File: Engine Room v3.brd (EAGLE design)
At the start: 72.4 x 35.6 mm, 28 parts, among them Q201 IRF6718, Q202 IRF6718, U101 PC847, U201 L298

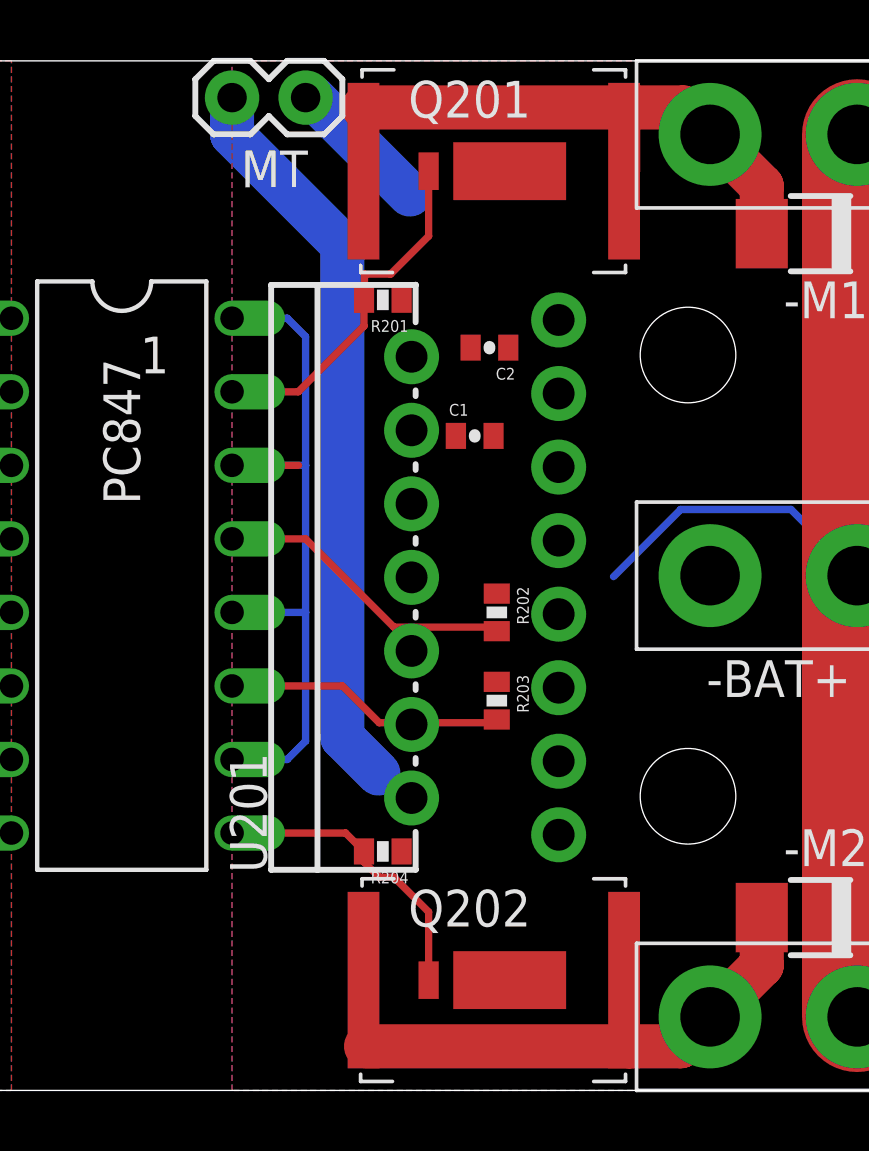
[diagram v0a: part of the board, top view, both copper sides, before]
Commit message: Added KwanAstro after the little crash of 2012
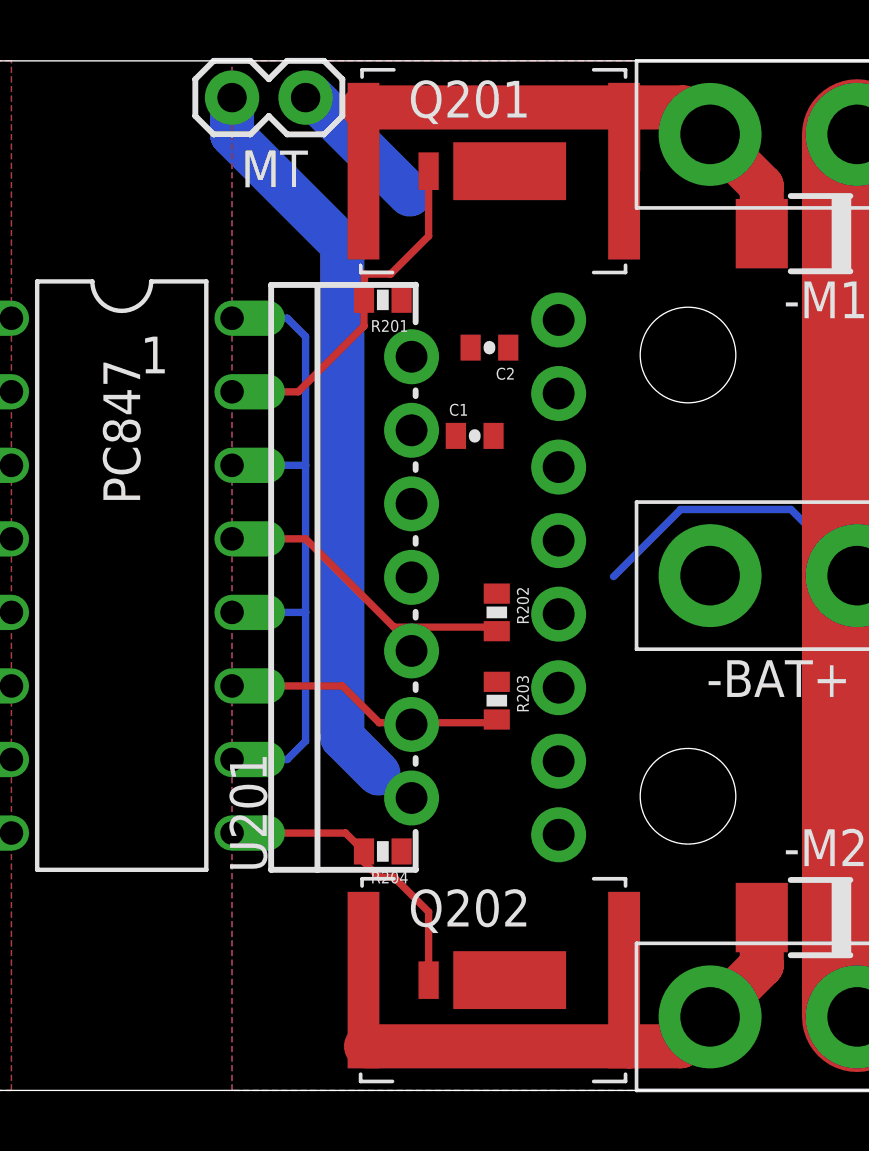
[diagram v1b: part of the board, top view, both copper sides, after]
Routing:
- net VDD: track 74.4 -> 72.1 mm
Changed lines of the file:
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@@
 <wire x1="64.77" y1="33.02" x2="66.555" y2="31.235" width="1.524" layer="1"/>
 <wire x1="66.555" y1="31.235" x2="66.555" y2="29.591" width="1.524" layer="1"/>
+<wire x1="63.84" y1="33.95" x2="62.23" y2="33.95" width="1.524" layer="1"/>
+<wire x1="62.23" y1="33.95" x2="52.8" y2="33.95" width="1.524" layer="1"/>
+<wire x1="62.23" y1="31.75" x2="62.23" y2="33.95" width="0.254" layer="1"/>
 <contactref element="Q201" pad="D1"/>
 <contactref element="Q201" pad="D2"/>
-<wire x1="63.84" y1="33.95" x2="62.23" y2="33.95" width="1.524" layer="1"/>
-<wire x1="62.23" y1="33.95" x2="52.8" y2="33.95" width="1.524" layer="1"/>
-<wire x1="52.8" y1="33.95" x2="52.8" y2="31.75" width="0.254" layer="1"/>
-<wire x1="61.8" y1="31.75" x2="62.23" y2="31.75" width="0.254" layer="1"/>
-<wire x1="62.23" y1="31.75" x2="62.23" y2="33.95" width="0.254" layer="1"/>
+<wire x1="52.8" y1="33.95" x2="53.34" y2="33.95" width="0.254" layer="1"/>
+<wire x1="53.34" y1="33.95" x2="53.34" y2="34.29" width="0.254" layer="1"/>
+<wire x1="52.8" y1="31.75" x2="52.8" y2="33.95" width="0.254" layer="1"/>
+<wire x1="62.23" y1="31.75" x2="61.8" y2="31.75" width="0" layer="19" extent="1-1"/>
 </signal>
 <signal name="M2-" class="1">
@@
 <wire x1="64.77" y1="2.54" x2="66.555" y2="4.325" width="1.524" layer="1"/>
 <wire x1="66.555" y1="4.325" x2="66.555" y2="5.969" width="1.524" layer="1"/>
+<wire x1="52.886" y1="1.524" x2="52.8" y2="1.524" width="0.254" layer="1"/>
+<wire x1="61.89" y1="3.81" x2="61.89" y2="1.61" width="0.254" layer="1"/>
 <contactref element="Q202" pad="D1"/>
 <contactref element="Q202" pad="D2"/>
-<wire x1="52.886" y1="1.524" x2="52.8" y2="1.524" width="0.254" layer="1"/>
 <wire x1="52.8" y1="1.524" x2="52.8" y2="3.81" width="0.254" layer="1"/>
-<wire x1="61.8" y1="3.81" x2="61.89" y2="3.81" width="0.254" layer="1"/>
-<wire x1="61.89" y1="3.81" x2="61.89" y2="1.61" width="0.254" layer="1"/>
+<wire x1="61.89" y1="3.81" x2="61.8" y2="3.81" width="0" layer="19" extent="1-1"/>
 </signal>
 <signal name="VDD" class="1">
@@
 <wire x1="69.85" y1="17.78" x2="67.564" y2="20.066" width="0.254" layer="16"/>
 <wire x1="69.85" y1="29.718" x2="69.462" y2="29.718" width="1.524" layer="1"/>
-<wire x1="48.26" y1="21.59" x2="50.557" y2="21.59" width="0.254" layer="1"/>
 <wire x1="50.8" y1="21.59" x2="48.26" y2="21.59" width="0.254" layer="16"/>
 <wire x1="69.85" y1="29.718" x2="69.977" y2="29.591" width="1.524" layer="1"/>
@@
 <wire x1="53.736" y1="28.194" x2="55.05" y2="29.508" width="0.254" layer="1"/>
 <contactref element="Q201" pad="G"/>
-<wire x1="55.05" y1="29.508" x2="55.05" y2="31.75" width="0.254" layer="1"/>
+<wire x1="55.05" y1="31.75" x2="55.05" y2="29.508" width="0.254" layer="1"/>
 </signal>
 <signal name="N$8">
@@
 <wire x1="52.817" y1="8.255" x2="52.817" y2="7.889" width="0.254" layer="1"/>
 <contactref element="Q202" pad="G"/>
-<wire x1="55.05" y1="6.164" x2="55.05" y2="3.81" width="0.254" layer="1"/>
+<wire x1="55.05" y1="3.81" x2="55.05" y2="6.164" width="0.254" layer="1"/>
 </signal>
 <signal name="N$10">
